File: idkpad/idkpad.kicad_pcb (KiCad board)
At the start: 2 copper layers, 41 parts, among them J1 Conn_01x02_Pin, J2 USB_C_Receptacle_USB2.0_16P, SW1 SW_DIP_x01, SW10 SW_DIP_x01, SW11 SW_DIP_x01, SW13 SW_DIP_x01, SW14 SW_DIP_x01, SW15 SW_DIP_x01, SW17 RotaryEncoder_Switch, SW19 RotaryEncoder_Switch, SW2 SW_DIP_x01, SW3 SW_DIP_x01, SW5 SW_DIP_x01, SW6 SW_DIP_x01, SW7 SW_DIP_x01, SW9 SW_DIP_x01, U1 ESP32-C3, U2 AMS1117-3.3, U3 USB6B1, Y1 Crystal_GND24_Small

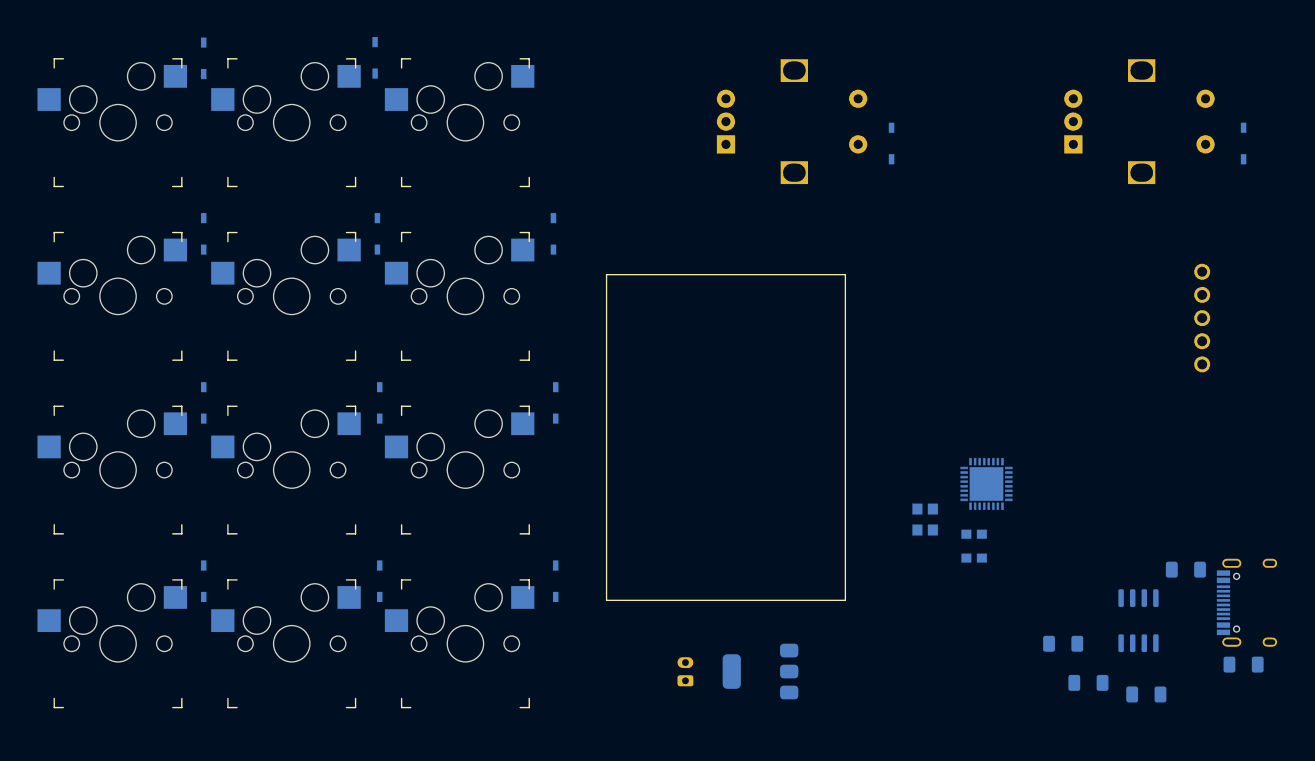
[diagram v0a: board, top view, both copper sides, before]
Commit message: bonk
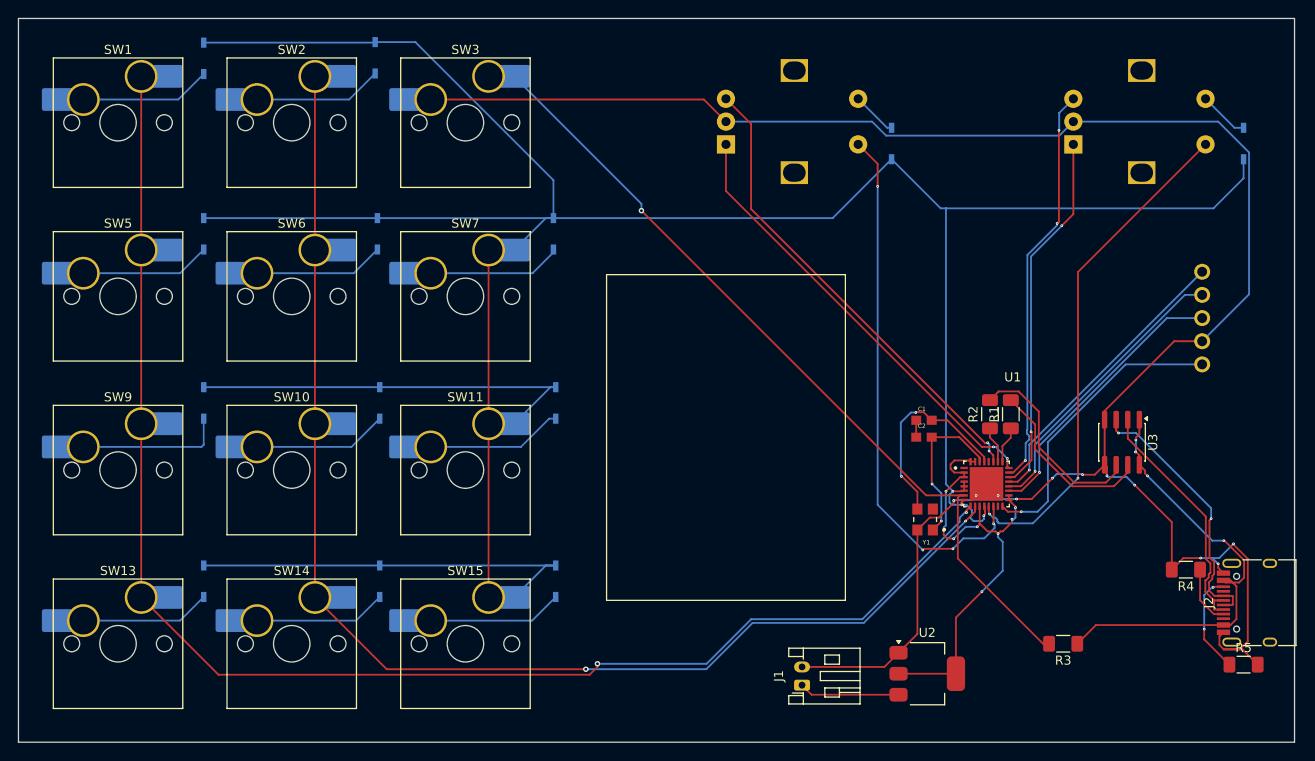
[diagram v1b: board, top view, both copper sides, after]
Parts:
- C1, C2, J1, J2, R1, R2, R3, R4, R5, U1, U2, U3, Y1: moved to F.Cu
- SW1, SW10, SW11, SW13, SW14, SW15, SW2, SW3, SW5, SW6, SW7, SW9: footprint kailh:Kailh_socket_MX -> PCM_Switch_Keyboard_Hotswap_Kailh:SW_Hotswap_Kailh_MX_Plated_1.00u
- moved R2 35.2 mm to (152.8, 89.1), turned to 90 degrees
- moved R1 30.7 mm to (155.1, 89.1), turned to 90 degrees
- moved U3 19.6 mm to (167.3, 92.2)
- moved U2 18.3 mm to (145.9, 117.6), turned to 0 degrees
- moved C2 14.4 mm to (145.5, 91.6), turned to 0 degrees
- moved C1 13.7 mm to (145.5, 89.8), turned to 0 degrees
- moved J1 12.8 mm to (132.2, 118.8)
- turned J2 to 90 degrees
- turned R4 to 180 degrees
- turned R5 to 0 degrees
- turned U1 to 0 degrees
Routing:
- net C3: track 0.00 -> 347.2 mm, vias 0 -> 3
- net GND: track 0.00 -> 231.8 mm, vias 0 -> 11
- net C1: track 0.00 -> 159.9 mm, vias 0 -> 2
- net C2: track 0.00 -> 140.6 mm, vias 0 -> 2
- net Net-(U1-CHIP_EN): track 0.00 -> 90.2 mm, vias 0 -> 1
- net C5: track 0.00 -> 59.0 mm, vias 0 -> 4
- net C4: track 0.00 -> 55.6 mm, vias 0 -> 2
- net RE_B2: track 0.00 -> 52.2 mm, vias 0 -> 2
- net Net-(U1-VDD3P3_CPU): track 0.00 -> 52.1 mm, vias 0 -> 8
- net VBUS: track 0.00 -> 49.7 mm, vias 0 -> 4
- net RE_A2: track 0.00 -> 49.2 mm, vias 0 -> 2
- net RE_B1: track 0.00 -> 44.6 mm, vias 0 -> 3
- net RE_A1: track 0.00 -> 39.9 mm, vias 0 -> 2
- net CS: track 0.00 -> 32.6 mm, vias 0 -> 1
- net MOSI: track 0.00 -> 32.4 mm, vias 0 -> 1
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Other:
- board outline added: 140 x 79.4 mm
